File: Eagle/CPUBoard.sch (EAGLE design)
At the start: 19 parts, among them IC2 MAX232, IC3 MAX481CPA, X1 BUTTON_BOARD, X2 RELAY_BOARD, X3 RS-485, X4 DISPLAY, X5 RS-232, X6 MKDSN1,5/3-5,08, X7 MKDSN1,5/3-5,08

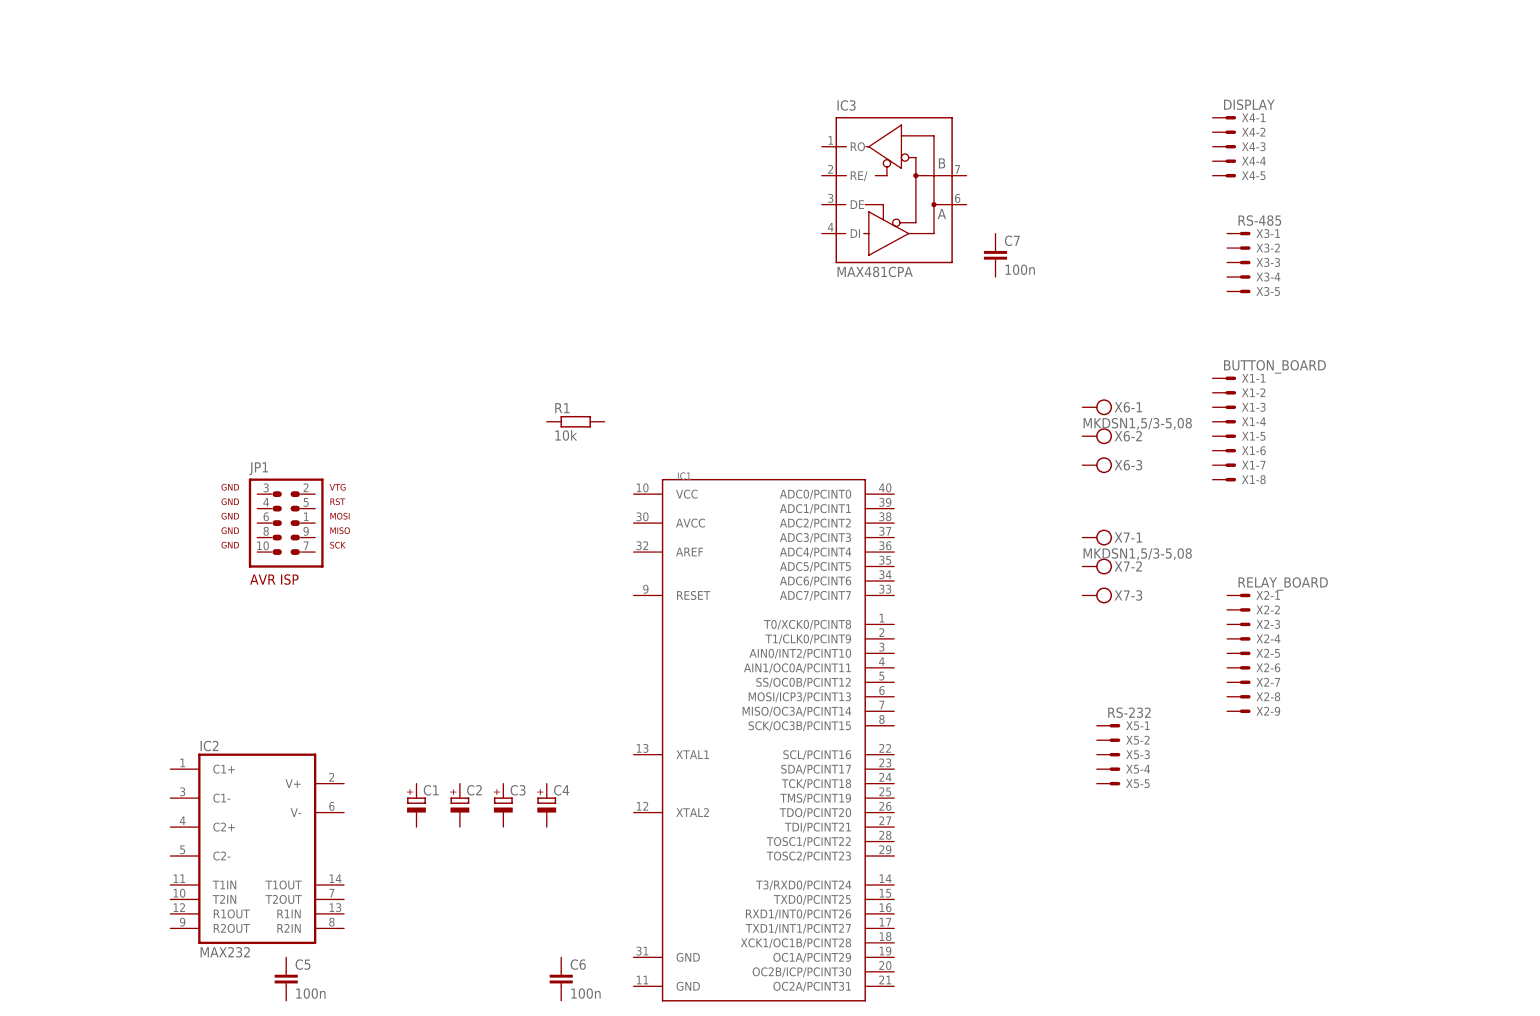
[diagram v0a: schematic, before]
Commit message: - more stuff added
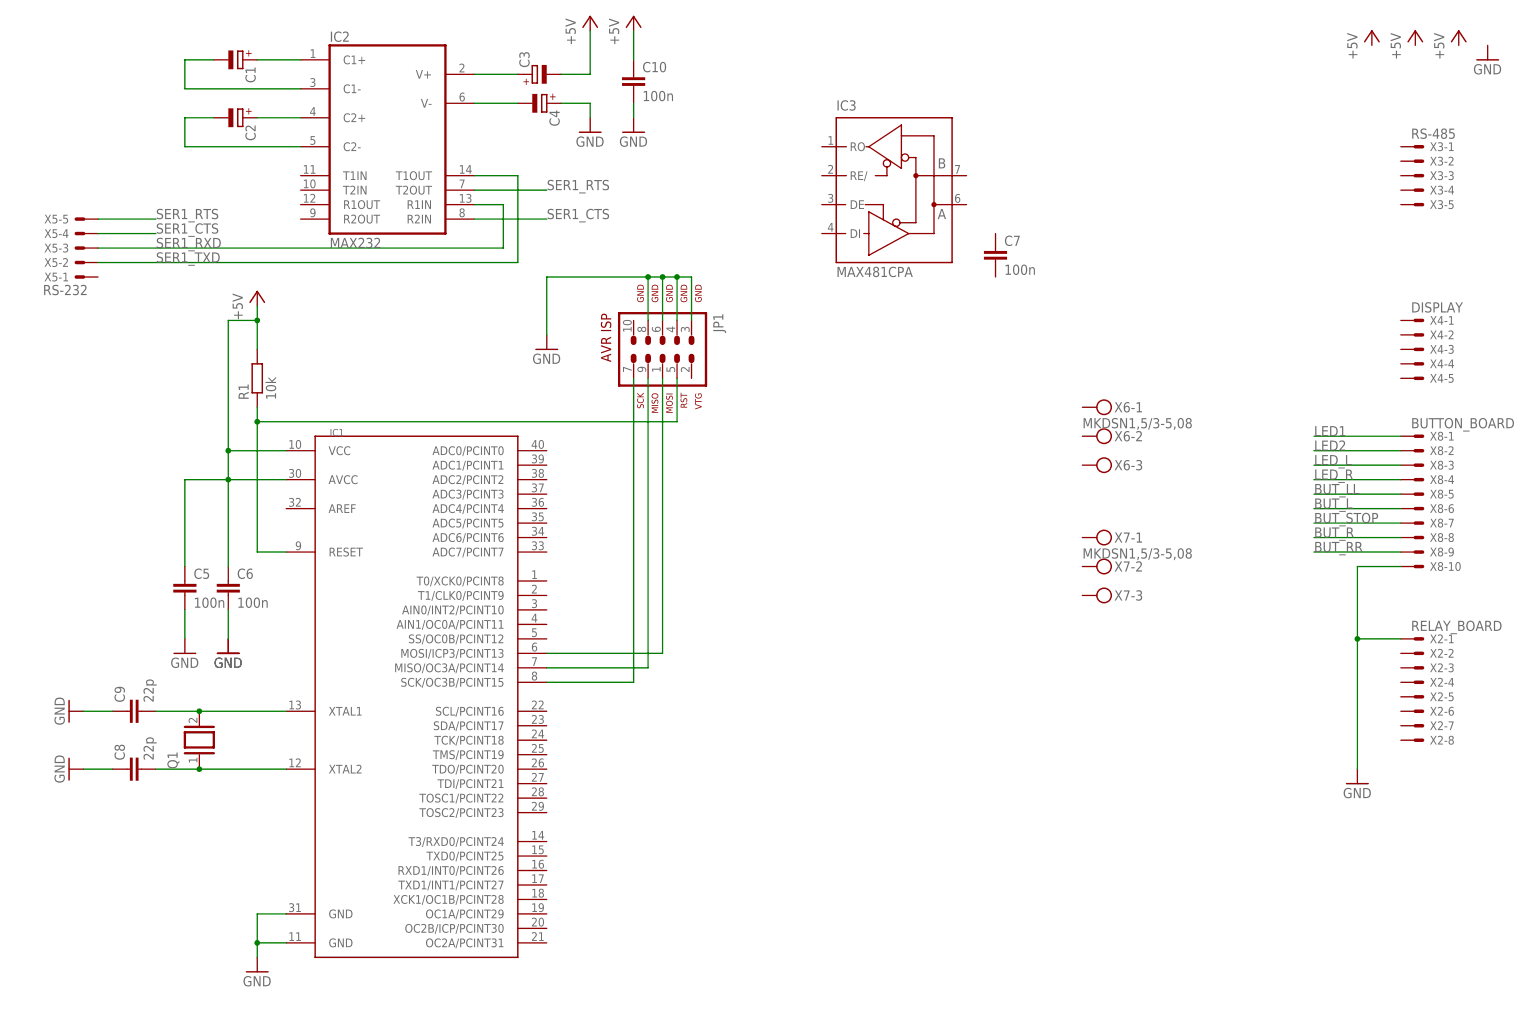
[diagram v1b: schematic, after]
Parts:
- removed X1: BUTTON_BOARD, con-molex:KK-156-8
- added C10: 100n, rcl:C-EU025-025X050
- added C8, C9: 22p, resistor:C-EU025-024X044
- added Q1: (no value), special:XTAL/S
- added X8: BUTTON_BOARD, con-molex:KK-156-10
- X2: device con-molex:KK-156-9 -> con-molex:KK-156-8
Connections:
- new net +5V: C10.1, C3.-, C5.1, C6.1, IC1.AVCC, IC1.VCC, R1.2
- new net BUT_L: X8-6.S
- new net BUT_LL: X8-5.S
- new net BUT_R: X8-8.S
- new net BUT_RR: X8-9.S
- new net BUT_STOP: X8-7.S
- new net GND: C10.2, C4.+, C5.2, C6.2, C8.1, C9.1, IC1.GND@0, IC1.GND@1, JP1.3, JP1.4, JP1.6, JP1.8, X2-1.S, X8-10.S
- new net LED1: X8-1.S
- new net LED2: X8-2.S
- new net LED_L: X8-3.S
- new net LED_R: X8-4.S
- new net N$1: C9.2, IC1.XTAL1, Q1.2
- new net N$10: C4.-, IC2G$1.V-
- new net N$11: IC1.SCK/OC3B/PCINT15, JP1.7
- new net N$13: IC1.MISO/OC3A/PCINT14, JP1.9
- new net N$14: IC1.MOSI/ICP3/PCINT13, JP1.1
- new net N$2: C8.2, IC1.XTAL2, Q1.1
- new net N$3: IC1.RESET, JP1.5, R1.1
- new net N$5: C1.+, IC2G$1.C1+
- new net N$6: C1.-, IC2G$1.C1-
- new net N$7: C2.+, IC2G$1.C2+
- new net N$8: C2.-, IC2G$1.C2-
- new net N$9: C3.+, IC2G$1.V+
- new net SER1_CTS: IC2G$1.R2IN, X5-4.S
- new net SER1_RTS: IC2G$1.T2OUT, X5-5.S
- new net SER1_RXD: IC2G$1.R1IN, X5-3.S
- new net SER1_TXD: IC2G$1.T1OUT, X5-2.S
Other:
- moved on the sheet: C1, C2, C3, C4, C5, C6, IC1, IC2, JP1, R1, X2-1, X2-2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

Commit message: - CPUBoard near final ...
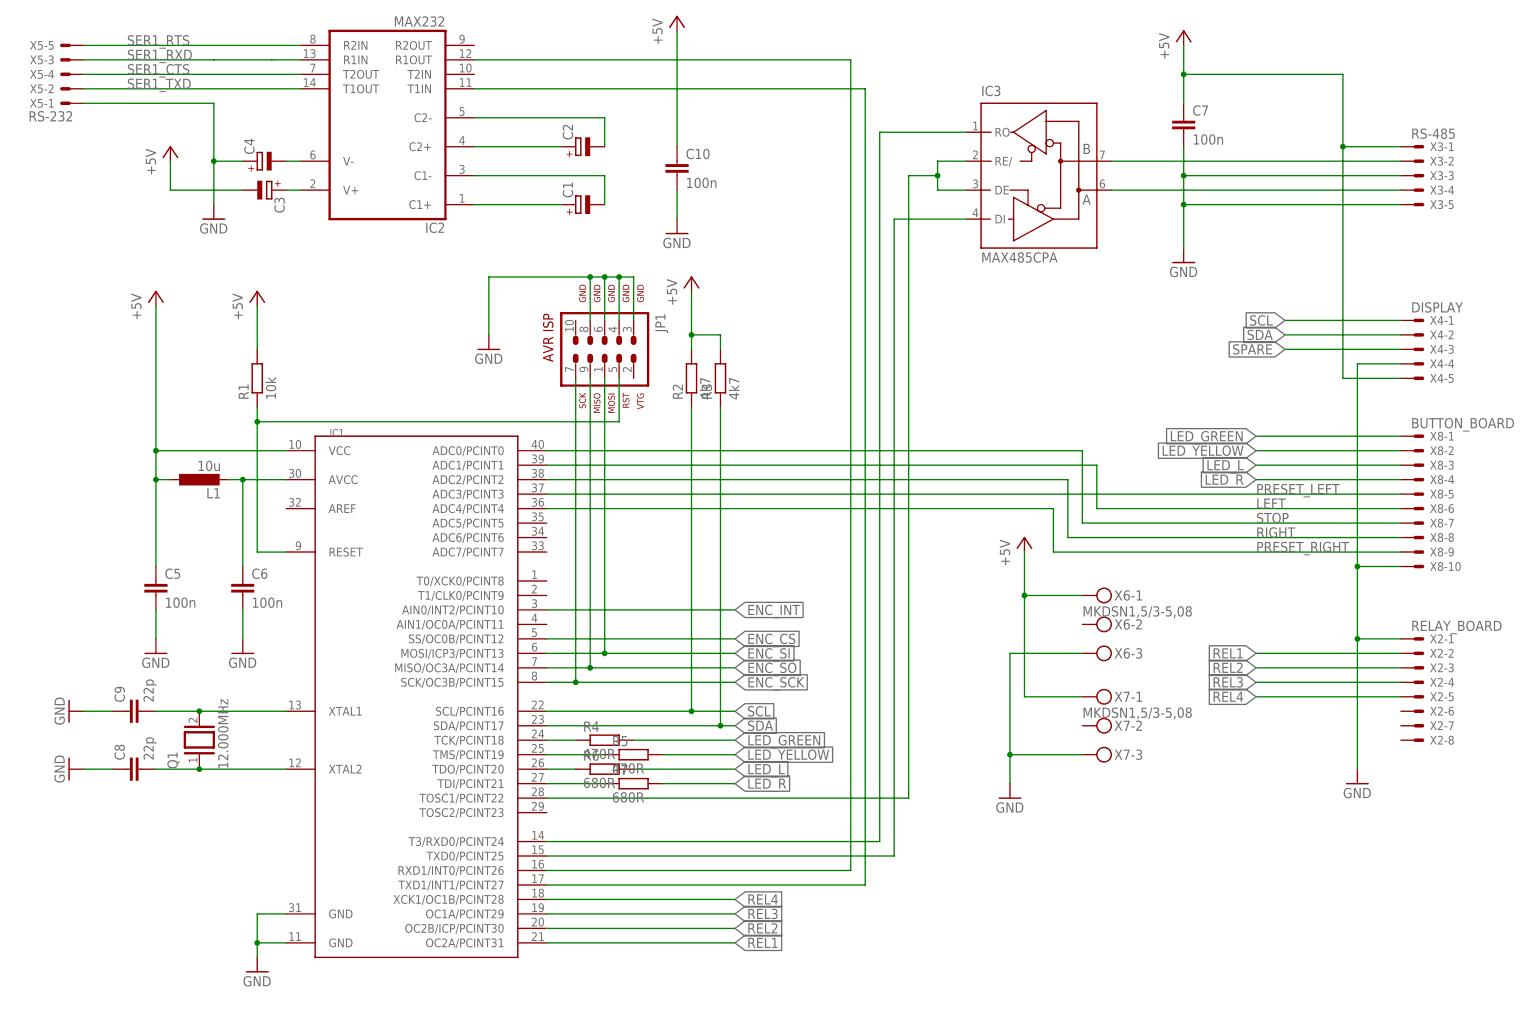
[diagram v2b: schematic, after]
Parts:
- added L1: 10u, rcl:L-EU0207/10
- added R2, R3: 4k7, rcl:R-EU_0207/10
- added R4, R5: 470R, rcl:R-EU_0207/10
- added R6, R7: 680R, rcl:R-EU_0207/10
- IC3: value MAX481CPA -> MAX485CPA
- Q1: value (none) -> 12.000MHz
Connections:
- net N$11 renamed ENC_SCK
- net N$13 renamed ENC_SO
- net N$14 renamed ENC_SI
- removed net BUT_L: X8-6.S
- removed net BUT_LL: X8-5.S
- removed net BUT_R: X8-8.S
- removed net BUT_RR: X8-9.S
- removed net BUT_STOP: X8-7.S
- removed net LED1: X8-1.S
- removed net LED2: X8-2.S
- new net ENC_CS: IC1.SS/OC0B/PCINT12
- new net ENC_INT: IC1.AIN0/INT2/PCINT10
- new net LED_GREEN: R4.2, X8-1.S
- new net LED_YELLOW: R5.2, X8-2.S
- new net LEFT: IC1.ADC1/PCINT1, X8-6.S
- new net N$11: IC1.RXD1/INT0/PCINT26, IC2G$1.R1OUT
- new net N$12: C6.1, IC1.AVCC, L1.2
- new net N$13: IC1.T3/RXD0/PCINT24, IC3G$1.RO
- new net N$14: IC1.TXD0/PCINT25, IC3G$1.DI
- new net N$15: IC1.TOSC1/PCINT22, IC3G$1.DE, IC3G$1.RE/
- new net N$17: IC3G$1.A, X3-4.S
- new net N$18: IC3G$1.B, X3-2.S
- new net N$20: IC1.TCK/PCINT18, R4.1
- new net N$21: IC1.TMS/PCINT19, R5.1
- new net N$22: IC1.TDO/PCINT20, R6.1
- new net N$23: IC1.TDI/PCINT21, R7.1
- new net N$4: IC1.TXD1/INT1/PCINT27, IC2G$1.T1IN
- new net PRESET_LEFT: IC1.ADC3/PCINT3, X8-5.S
- new net PRESET_RIGHT: IC1.ADC4/PCINT4, X8-9.S
- new net REL1: IC1.OC2A/PCINT31, X2-2.S
- new net REL2: IC1.OC2B/ICP/PCINT30, X2-3.S
- new net REL3: IC1.OC1A/PCINT29, X2-4.S
- new net REL4: IC1.XCK1/OC1B/PCINT28, X2-5.S
- new net RIGHT: IC1.ADC2/PCINT2, X8-8.S
- new net SCL: IC1.SCL/PCINT16, R2.1, X4-1.S
- new net SDA: IC1.SDA/PCINT17, R3.1, X4-2.S
- new net SPARE: X4-3.S
- new net STOP: IC1.ADC0/PCINT0, X8-7.S
- net +5V: now also C7.1, L1.1, R2.2, R3.2, X3-1.S, X4-5.S, X6-1.KL, X7-1.KL; no longer C6.1, IC1.AVCC
- net GND: now also C7.2, X3-3.S, X3-5.S, X4-4.S, X5-1.S, X6-3.KL, X7-3.KL
- net LED_L: now also R6.2
- net LED_R: now also R7.2
- net SER1_CTS: now also IC2G$1.T2OUT; no longer IC2G$1.R2IN
- net SER1_RTS: now also IC2G$1.R2IN; no longer IC2G$1.T2OUT
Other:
- moved on the sheet: C1, C10, C2, C3, C4, C5, C6, C7, IC2, IC3, JP1, X5-1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
